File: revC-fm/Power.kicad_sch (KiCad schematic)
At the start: 70 parts, among them P2 TSM-102-01-L-SV-P-TR, Q1 MMDT5551-7-F, Q2 MMDT5551-7-F, Q28 MMDT5551-7-F, SW3 SW_SPST, SW4 SW_SPST, SW5 SW_SPST, SW6 SW_SPST, U11 INA230AIRGTR, U12 INA230AIRGTR, U13 INA230AIRGTR, U14 INA230AIRGTR, U15 BQ25883RGER, U16 TPS54226PWPR, U17 INA230AIRGTR

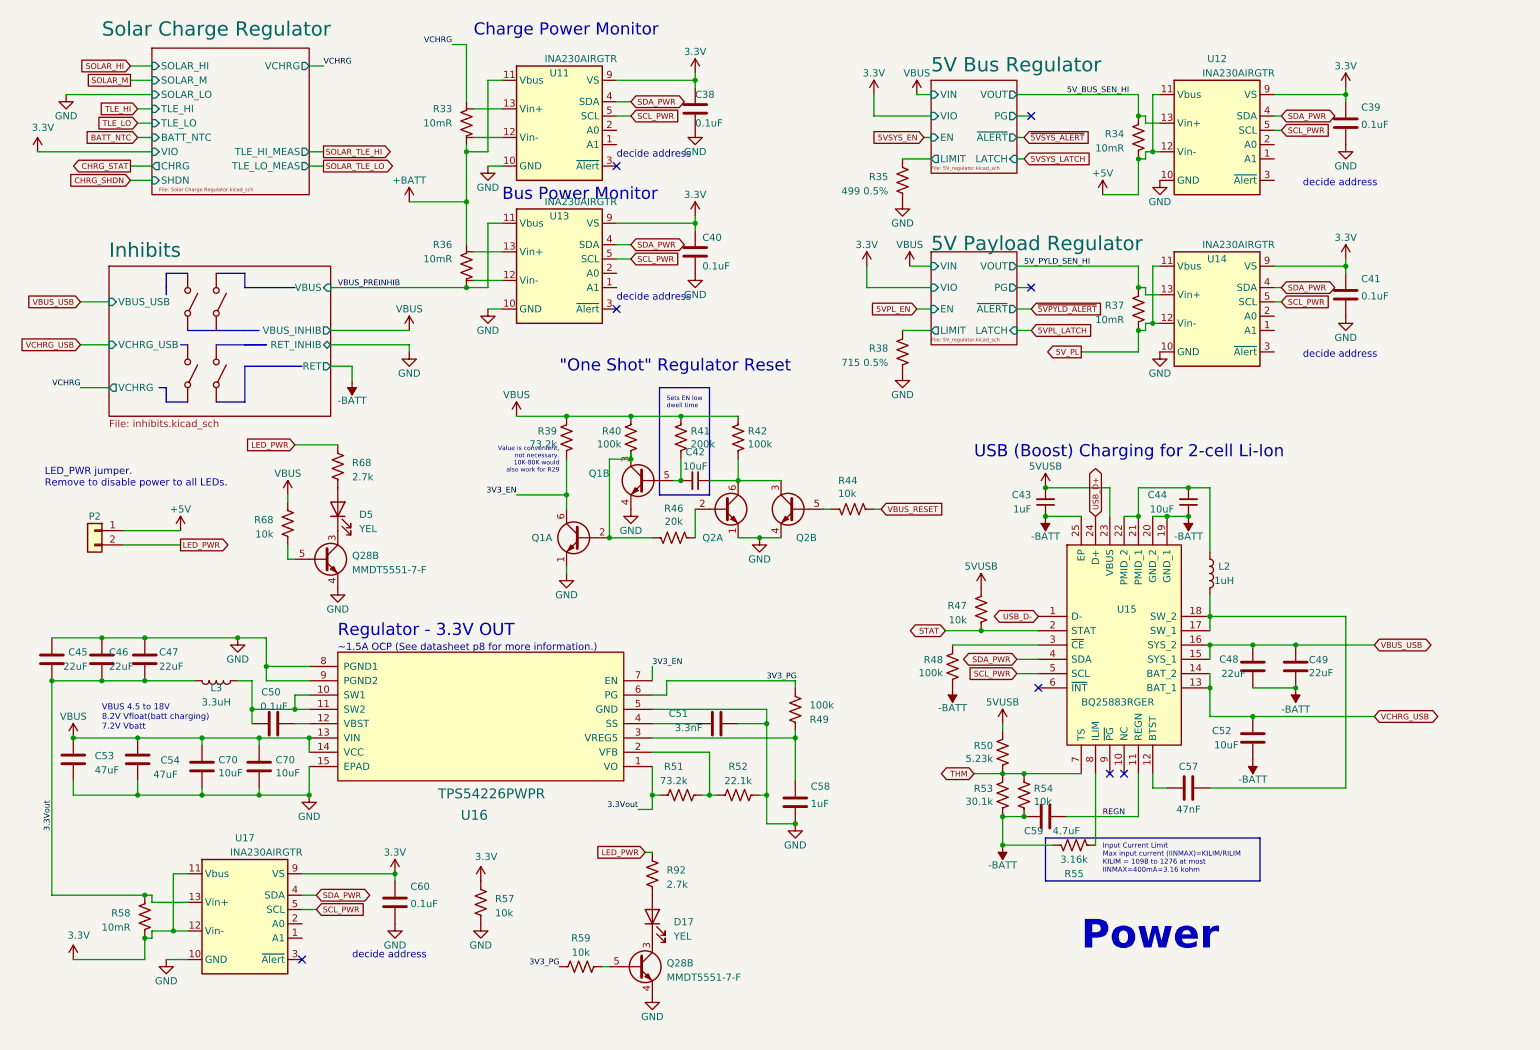
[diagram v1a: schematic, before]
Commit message: working revC
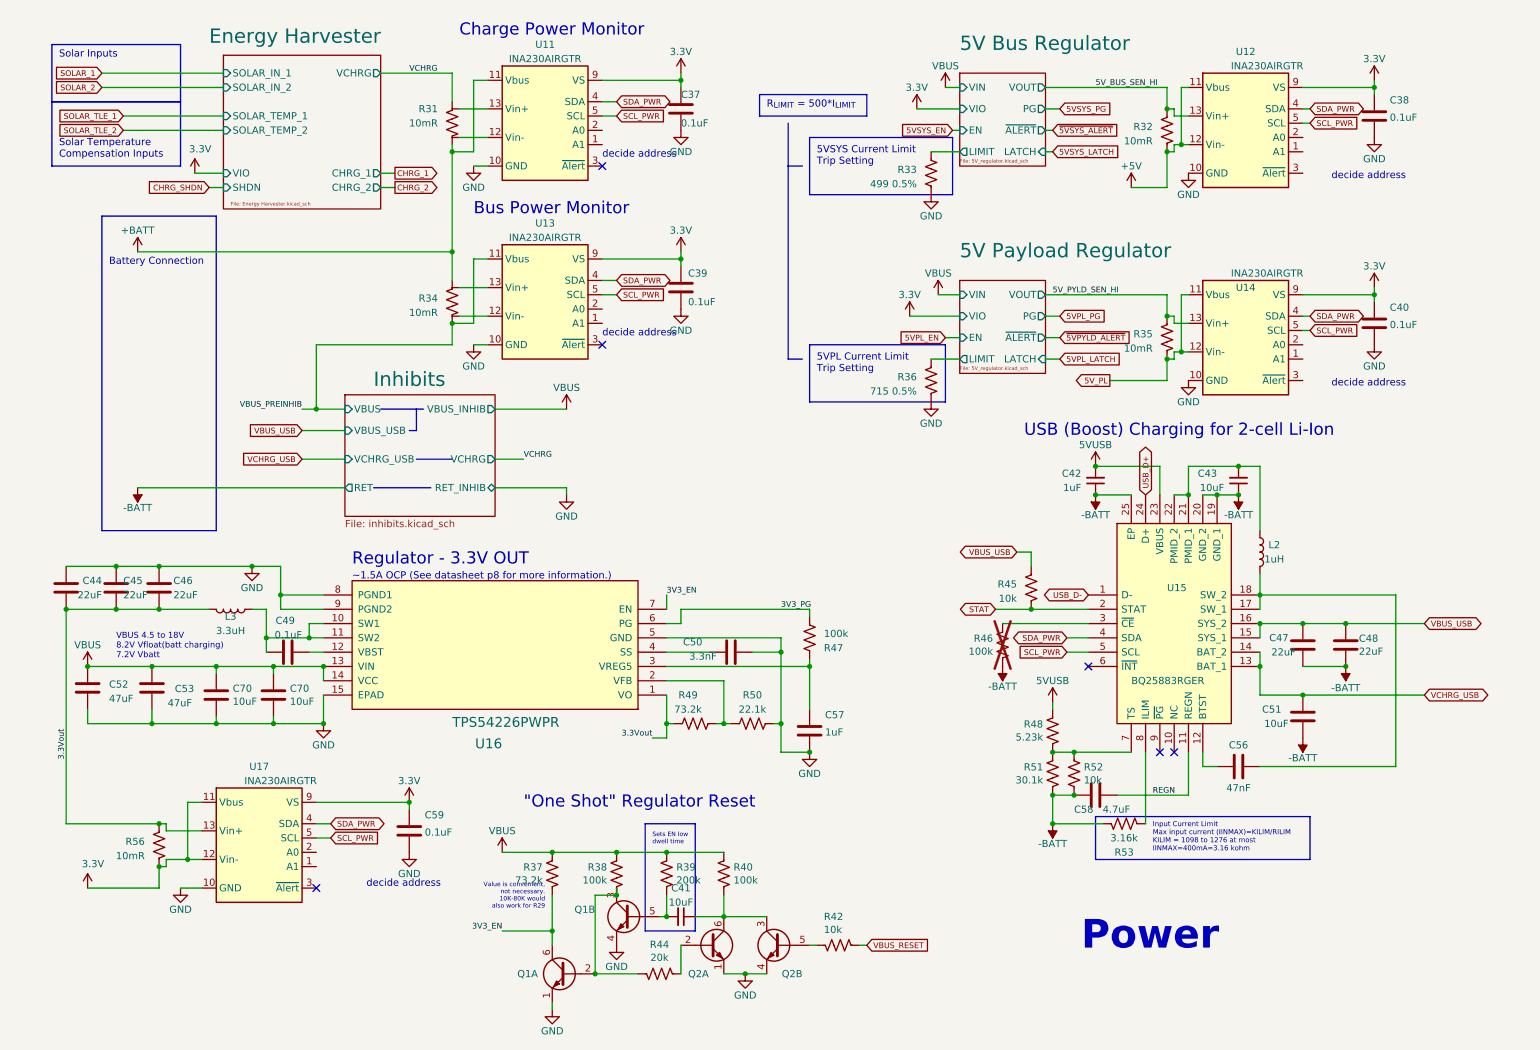
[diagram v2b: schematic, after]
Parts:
- removed D17, D5: YEL, LED_SMD:LED_0603_1608Metric, symbol Device:LED
- removed P2: TSM-102-01-L-SV-P-TR, Connector_PinHeader_2.54mm:PinHeader_1x02_P2.54mm_Vertical_SMD_Pin1Right, symbol Connector_Generic:Conn_01x02
- removed Q28 (x2): MMDT5551-7-F, Package_TO_SOT_SMD:SOT-363_SC-70-6, symbol Transistor_BJT:MMDT5551
- removed R57, R59, R68: 10k, Resistor_SMD:R_0603_1608Metric, symbol Device:R_US
- removed R68, R92: 2.7k, Resistor_SMD:R_0603_1608Metric, symbol Device:R_US
- removed SW3, SW4, SW5, SW6: SW_SPST, symbol Switch:SW_SPST
- C37: renamed from C38; footprint Capacitor_SMD:C_0603_1608Metric -> Capacitor_SMD:C_0402_1005Metric
- C38: renamed from C39; footprint Capacitor_SMD:C_0603_1608Metric -> Capacitor_SMD:C_0402_1005Metric
- C39: renamed from C40; footprint Capacitor_SMD:C_0603_1608Metric -> Capacitor_SMD:C_0402_1005Metric
- C40: renamed from C41; footprint Capacitor_SMD:C_0603_1608Metric -> Capacitor_SMD:C_0402_1005Metric
- C41: renamed from C42; Mfr. Part No (none) -> CGA4J1X7S1E106K125AE
- C43: renamed from C44; Mfr. Part No (none) -> CGA4J1X7S1E106K125AE
- C44: renamed from C45; Mfr. Part No (none) -> GRT21BR61C226ME13K
- C45: renamed from C46; Mfr. Part No (none) -> GRT21BR61C226ME13K
- C46: renamed from C47; Mfr. Part No (none) -> GRT21BR61C226ME13K
- C47: renamed from C48; Mfr. Part No (none) -> GRT21BR61C226ME13K
- C48: renamed from C49; Mfr. Part No (none) -> GRT21BR61C226ME13K
- C49: renamed from C50; footprint Capacitor_SMD:C_0603_1608Metric -> Capacitor_SMD:C_0402_1005Metric
- C50: renamed from C51; footprint Capacitor_SMD:C_0603_1608Metric -> Capacitor_SMD:C_0402_1005Metric
- C51: renamed from C52; Mfr. Part No (none) -> CGA4J1X7S1E106K125AE
- C52: renamed from C53; Mfr. Part No (none) -> C3216X5R1E476M160AC
- C53: renamed from C54; Mfr. Part No (none) -> C3216X5R1E476M160AC
- C56: renamed from C57; footprint Capacitor_SMD:C_0603_1608Metric -> Capacitor_SMD:C_0402_1005Metric
- C58: renamed from C59; footprint Capacitor_SMD:C_0805_2012Metric -> Capacitor_SMD:C_0603_1608Metric
- C59: renamed from C60; footprint Capacitor_SMD:C_0603_1608Metric -> Capacitor_SMD:C_0402_1005Metric
- C70: Mfr. Part No (none) -> CGA4J1X7S1E106K125AE
- L2: Mfr. Part No (none) -> 74404032010
- L3: Mfr. Part No (none) -> 744316330
- R31: renamed from R33; Mfr. Part No (none) -> KRL3216T4A-M-R010-F-T1
- R32: renamed from R34; footprint Resistor_SMD:R_1210_3225Metric -> Resistor_SMD:R_1206_3216Metric
- R34: renamed from R36; Mfr. Part No (none) -> KRL3216T4A-M-R010-F-T1
- R35: renamed from R37; footprint Resistor_SMD:R_1210_3225Metric -> Resistor_SMD:R_1206_3216Metric
- R38: renamed from R40; footprint Resistor_SMD:R_0603_1608Metric -> Resistor_SMD:R_0402_1005Metric
- R39: renamed from R41; footprint Resistor_SMD:R_0603_1608Metric -> Resistor_SMD:R_0402_1005Metric
- R40: renamed from R42; footprint Resistor_SMD:R_0603_1608Metric -> Resistor_SMD:R_0402_1005Metric
- R42: renamed from R44; footprint Resistor_SMD:R_0603_1608Metric -> Resistor_SMD:R_0402_1005Metric
- R44: renamed from R46; footprint Resistor_SMD:R_0603_1608Metric -> Resistor_SMD:R_0402_1005Metric
- R45: renamed from R47; footprint Resistor_SMD:R_0603_1608Metric -> Resistor_SMD:R_0402_1005Metric
- R46: renamed from R48; footprint Resistor_SMD:R_0603_1608Metric -> Resistor_SMD:R_0402_1005Metric; now not fitted
- R47: renamed from R49; footprint Resistor_SMD:R_0603_1608Metric -> Resistor_SMD:R_0402_1005Metric
- R52: renamed from R54; footprint Resistor_SMD:R_0603_1608Metric -> Resistor_SMD:R_0402_1005Metric
- U11, U12, U13, U14, U17: Mfr. Part No (none) -> INA230AIRGTR
- U15: Mfr. Part No (none) -> BQ25883RGER
- U16: Mfr. Part No (none) -> TPS54226PWPR
- renumbered C43 to C42, C58 to C57, R35 to R33, R38 to R36, R39 to R37, R50 to R48, R51 to R49, R52 to R50, R53 to R51, R55 to R53, R58 to R56
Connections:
- net 5VUSB: no longer R45.2
- net VBUS_USB: now also R45.2
- net THM: no longer names the net of R48.2, R51.2, R52.2, U15.7 (TS)
- no-connect marks 8 -> 6
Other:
- sheet Solar Charge Regulator renamed Energy Harvester
- sheet Energy Harvester: file Solar Charge Regulator.kicad_sch -> Energy Harvester.kicad_sch
- sheet Energy Harvester ports: added CHRG_1, CHRG_2, SOLAR_IN_1, SOLAR_IN_2, SOLAR_TEMP_1, SOLAR_TEMP_2; removed BATT_NTC, CHRG, SOLAR_HI, SOLAR_LO, SOLAR_M, TLE_HI, TLE_HI_MEAS, TLE_LO, TLE_LO_MEAS
- note added: "5VPL Current Limit Trip Setting"
- note added: "5VSYS Current Limit Trip Setting"
- note added: "Battery Connection"
- note added: "R_{LIMIT} = 500*I_{LIMIT}"
- note added: "Solar Inputs"
- note added: "Solar Temperature Compensation Inputs"
- note removed: "LED_PWR jumper. Remove to disable power to all LEDs."
- moved on the sheet: C37, C38, C39, C40, C41, C42, C43, C44, C45, C46, C47, C48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

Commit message: working
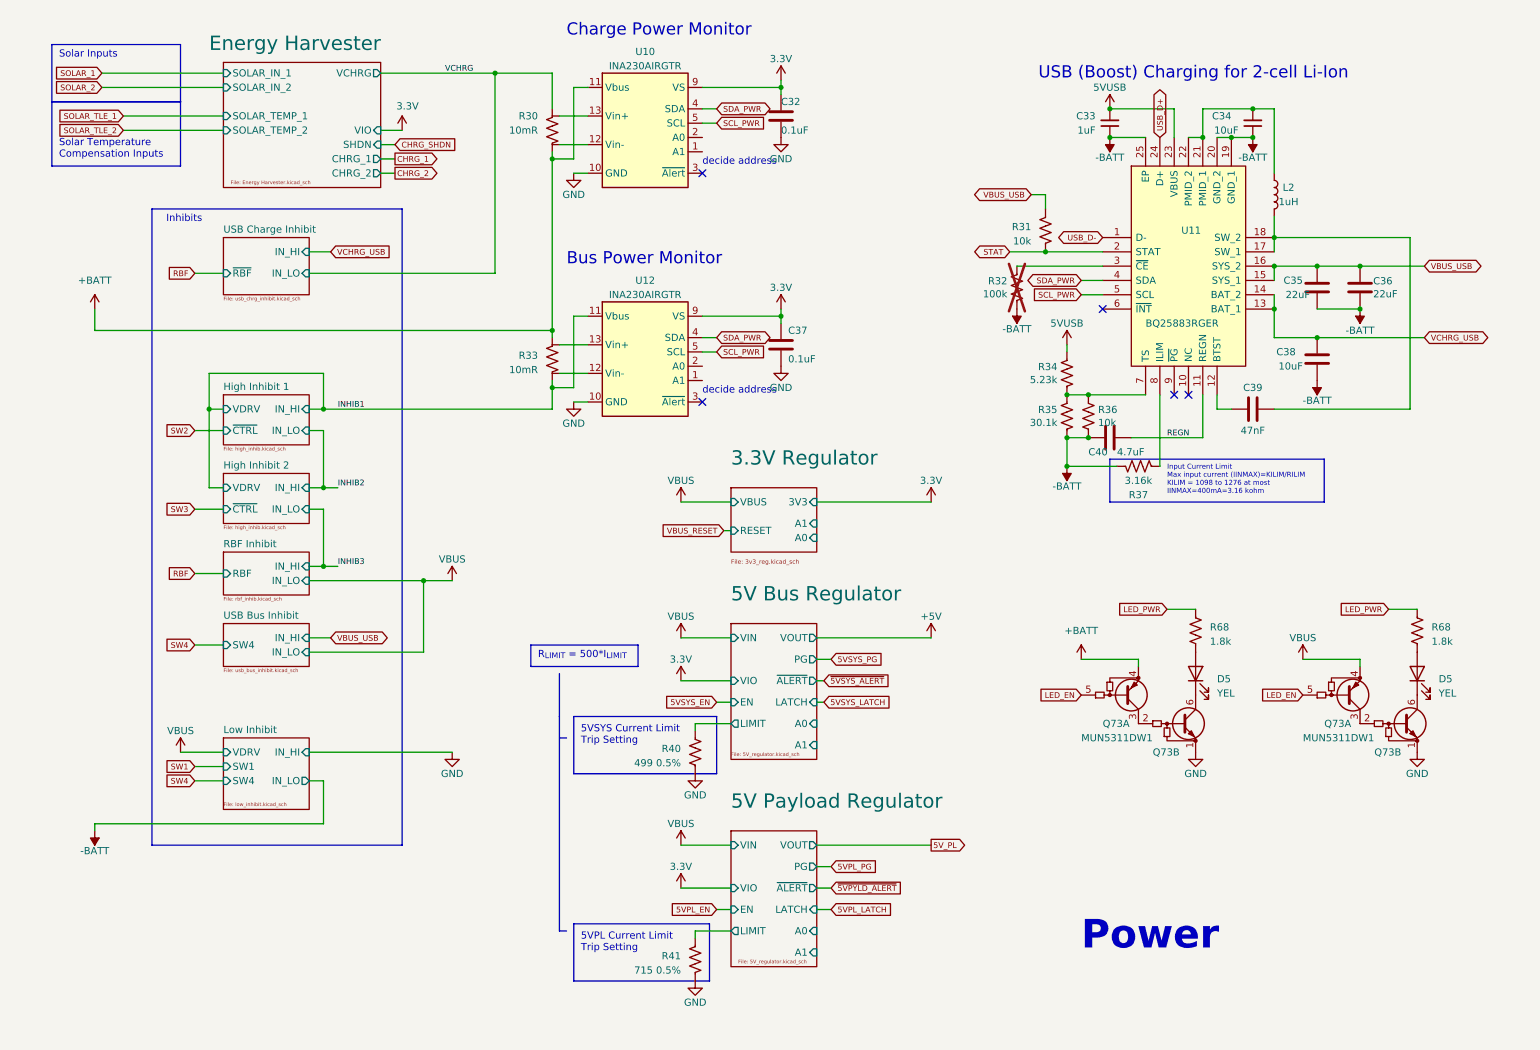
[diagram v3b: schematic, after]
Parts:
- removed C38, C40, C49, C59: 0.1uF, Capacitor_SMD:C_0402_1005Metric, symbol Device:C
- removed C41: 10uF, Capacitor_SMD:C_0805_2012Metric, symbol Device:C_Small
- removed C44, C45, C46: 22uF, Capacitor_SMD:C_0805_2012Metric, symbol Device:C
- removed C50: 3.3nF, Capacitor_SMD:C_0402_1005Metric, symbol Device:C
- removed C52, C53: 47uF, Capacitor_SMD:C_1206_3216Metric, symbol Device:C
- removed C57: 1uF, Capacitor_SMD:C_0603_1608Metric, symbol Device:C
- removed C70 (x2): 10uF, Capacitor_SMD:C_0805_2012Metric, symbol Device:C
- removed L3: 3.3uH, SierraLobo:L_Wuerth_HCI-5040, symbol Device:L
- removed Q1, Q2: MMDT5551-7-F, Package_TO_SOT_SMD:SOT-363_SC-70-6, symbol Transistor_BJT:MMDT5551
- removed R32, R35: 10mR, Resistor_SMD:R_1206_3216Metric, symbol Device:R_US
- removed R37, R49: 73.2k, Resistor_SMD:R_0603_1608Metric, symbol Device:R_US
- removed R38, R40, R47: 100k, Resistor_SMD:R_0402_1005Metric, symbol Device:R_US
- removed R39: 200k, Resistor_SMD:R_0402_1005Metric, symbol Device:R_US
- removed R42: 10k, Resistor_SMD:R_0402_1005Metric, symbol Device:R_US
- removed R44: 20k, Resistor_SMD:R_0402_1005Metric, symbol Device:R_US
- removed R50: 22.1k, Resistor_SMD:R_0603_1608Metric, symbol Device:R_US
- removed R56: 10mR, Resistor_SMD:R_1210_3225Metric, symbol Device:R_US
- removed U12, U14, U17: INA230AIRGTR, SierraLobo:INA230AIRGTR, symbol SierraLobo:INA230AxRGT
- removed U16: TPS54226PWPR, SierraLobo:PWP14_2P31X2P46-L, symbol SierraLobo:TPS54226PWPR
- added D5 (x2): YEL, LED_SMD:LED_0402_1005Metric, symbol Device:LED
- added Q73 (x2): MUN5311DW1, Package_TO_SOT_SMD:SOT-363_SC-70-6, symbol SierraLobo:MUN5312DW1
- added R68 (x2): 1.8k, Resistor_SMD:R_0402_1005Metric, symbol Device:R_US
- renumbered C37 to C32, C42 to C33, C43 to C34, C47 to C35, C48 to C36, C39 to C37, C51 to C38, C56 to C39, C58 to C40, R31 to R30, R45 to R31, R46 to R32, R34 to R33, R48 to R34, R51 to R35, R52 to R36, R53 to R37, R33 to R40, R36 to R41, U11 to U10, U15 to U11, U13 to U12
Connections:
- net +BATT: now also Q73.4 (E1)
- net EP: now also Q73.1 (E2), Q73.1 (E2)
- net VBUS: now also Q73.4 (E1)
- net VBUS_PREINHIB renamed INHIB1
- new net: Q73.2 (B2), Q73.3 (C1) (x2)
- new net: D5.1 (K), Q73.6 (C2) (x2)
- new net: D5.2 (A), R68.1 (x2)
- new net LED_EN: Q73.5 (B1), Q73.5 (B1)
- new net LED_PWR: R68.2, R68.2
- no-connect marks 6 -> 5
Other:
- removed sheet Inhibits
- added sheet 3.3V Regulator (3v3_reg.kicad_sch)
- added sheet High Inhibit 1 (high_inhib.kicad_sch)
- added sheet High Inhibit 2 (high_inhib.kicad_sch)
- added sheet Low Inhibit (low_inhibit.kicad_sch)
- added sheet RBF Inhibit (rbf_inhib.kicad_sch)
- added sheet USB Bus Inhibit (usb_bus_inhibit.kicad_sch)
- added sheet USB Charge Inhibit (usb_chrg_inhibit.kicad_sch)
- sheet 5V Bus Regulator ports: added A0, A1; removed none
- sheet 5V Payload Regulator ports: added A0, A1; removed none
- note added: "Inhibits"
- note removed: ""One Shot" Regulator Reset"
- note removed: "Battery Connection"
- note removed: "Regulator - 3.3V OUT"
- note removed: "Sets EN low dwell time"
- note removed: "VBUS 4.5 to 18V 8.2V Vfloat(batt charging) 7.2V Vbatt"
- note removed: "Value is convenient, not necessary. 10K-80K would also work for R29"
- note removed: "~1.5A OCP (See datasheet p8 for more information.)"
- moved on the sheet: C32, C33, C34, C35, C36, C37, C38, C39, C40, L2, R30, R31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
